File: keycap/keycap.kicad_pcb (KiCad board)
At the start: 2 copper layers, 15.5 x 15.5 mm, 14 parts, among them J1 Conn_01x01_Female, J10 Conn_01x01_Female, J2 Conn_01x01_Female, J3 Conn_01x01_Female, J4 Conn_01x01_Female, J5 Conn_01x01_Female, J6 Conn_01x01_Female, J7 Conn_01x01_Female, J8 Conn_01x01_Female, J9 Conn_01x01_Female, SW1 SW_Push_Open

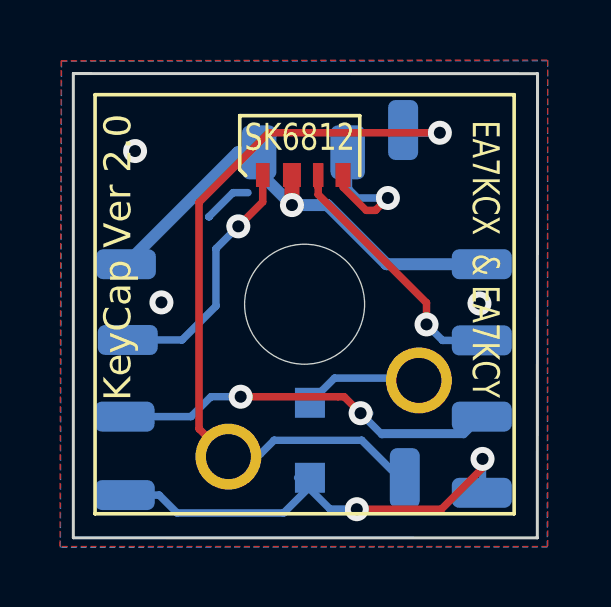
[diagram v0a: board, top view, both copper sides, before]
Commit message: Nueva rama develop
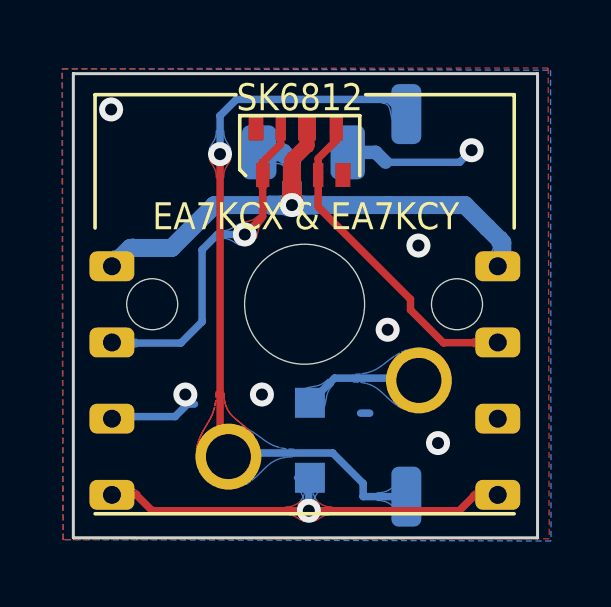
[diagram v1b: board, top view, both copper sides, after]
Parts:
- added REF**: SK6812, Battery:LED_SK6812_4020_, F.Cu at (120.7, 108.6)
- SW1: footprint Button_Switch_Keyboard:SW_Cherry_MX_1.00u_Plate -> Button_Switch_Keyboard:SW_Cherry_MX_1.00u_PCB
- moved J8 0.62 mm to (124.5, 119.7)
- moved J5 0.54 mm to (127.6, 114.6)
- moved J9 0.53 mm to (124.4, 106.9)
- moved J7 0.53 mm to (127.5, 119.7)
- moved J6 0.52 mm to (127.5, 117.1)
- moved J4 0.51 mm to (127.5, 112.0)
- moved J2 0.50 mm to (114.7, 114.5)
- moved J10 0.42 mm to (114.7, 119.6)
- moved J3 0.39 mm to (114.7, 117.0)
- moved J1 0.18 mm to (115.0, 112.0)
- renumbered C1 to C, D1 to D
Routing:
- net GND: track 18.8 -> 7.64 mm, vias 6 -> 7
- net /VCC: track 18.0 -> 23.1 mm
- net /DIN: track 8.52 -> 11.8 mm
- net /DOUT: track 8.95 -> 11.5 mm, vias 1 -> 0
- net (no net): track 1.65 -> 0.00 mm
- net /COL: track 25.9 -> 27.2 mm
- net /ROW: vias 2 -> 1
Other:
- rule trace_min: 0.2 -> 0.1
- rule via_min_size: 0.4 -> 0.2
- board text removed: "KeyCap Ver 2.0"
